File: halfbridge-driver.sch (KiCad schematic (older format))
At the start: 29 parts, among them U1 MGJ1, U2 2ED020I12-F2, U3 MGJ1

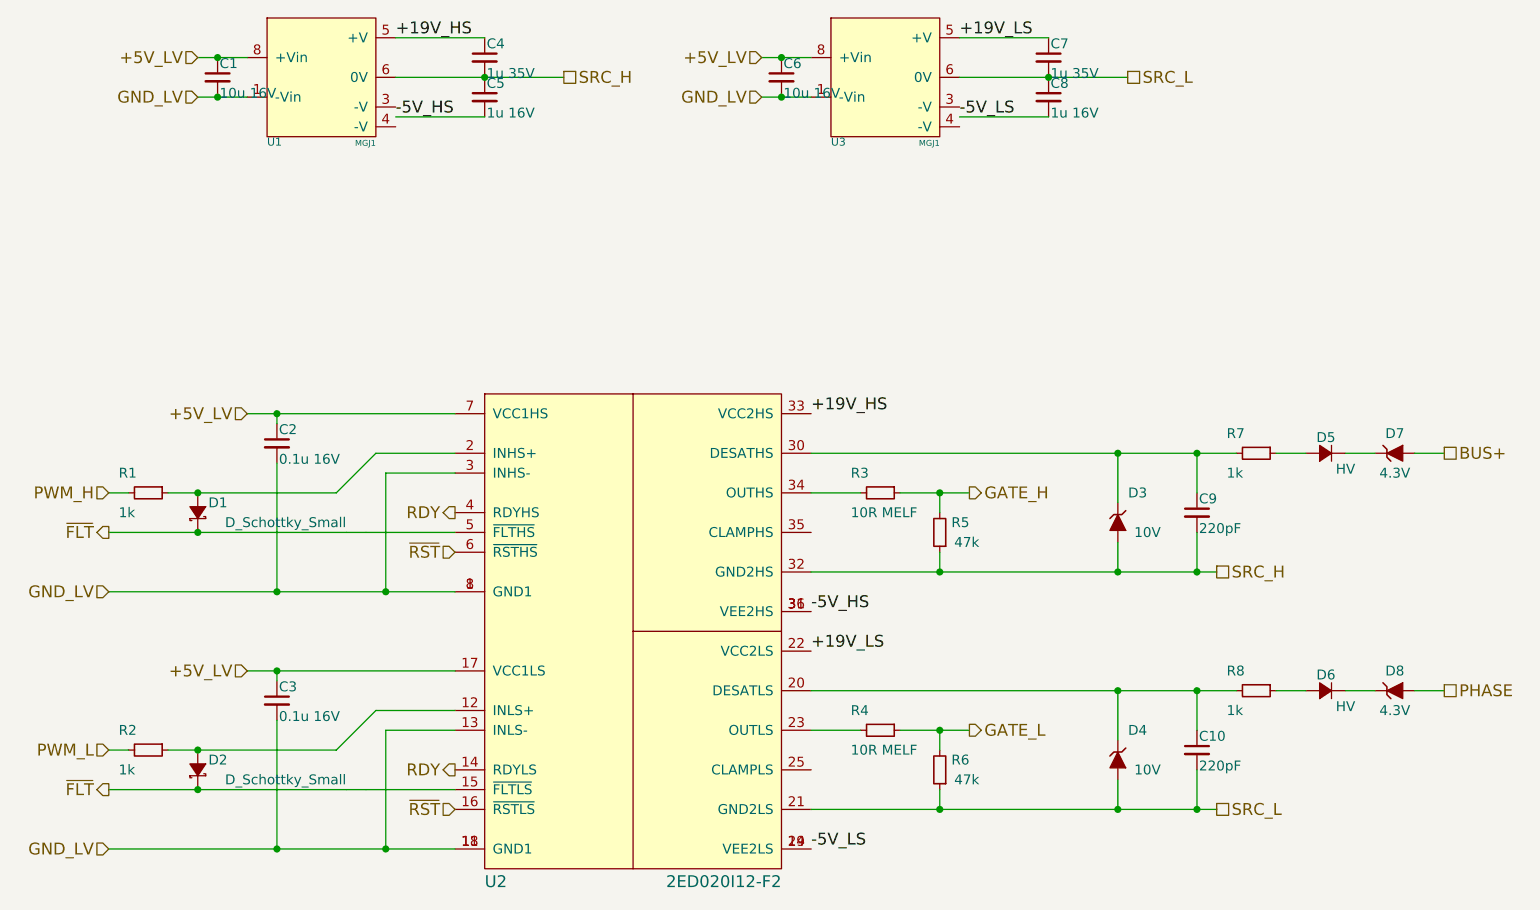
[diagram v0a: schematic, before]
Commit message: progress on V2 schematic
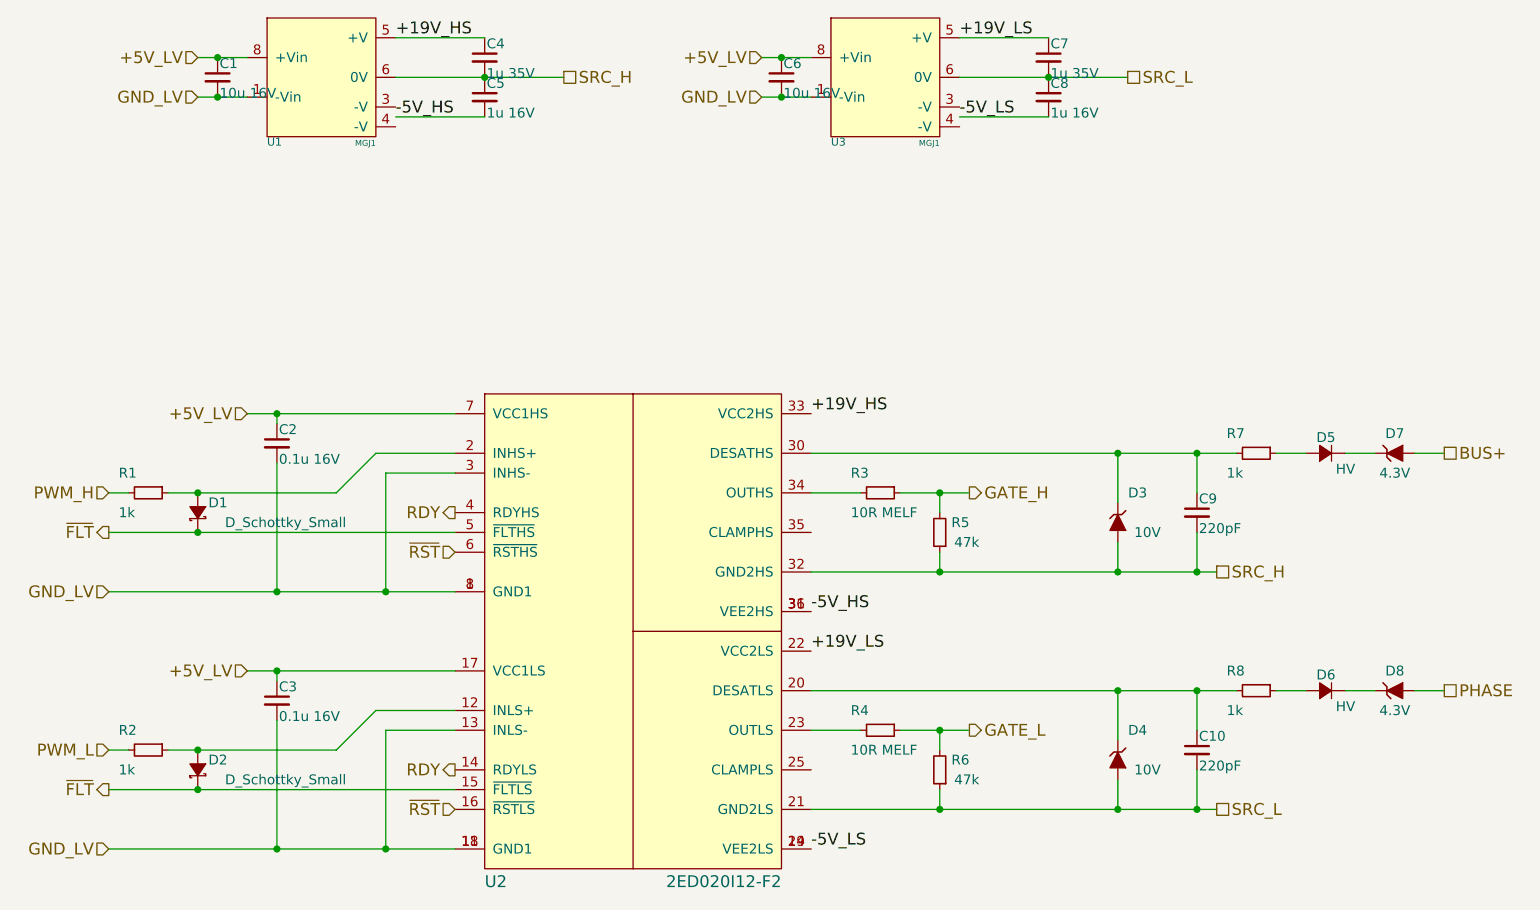
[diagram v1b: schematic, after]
